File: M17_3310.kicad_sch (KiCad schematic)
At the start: 0 parts

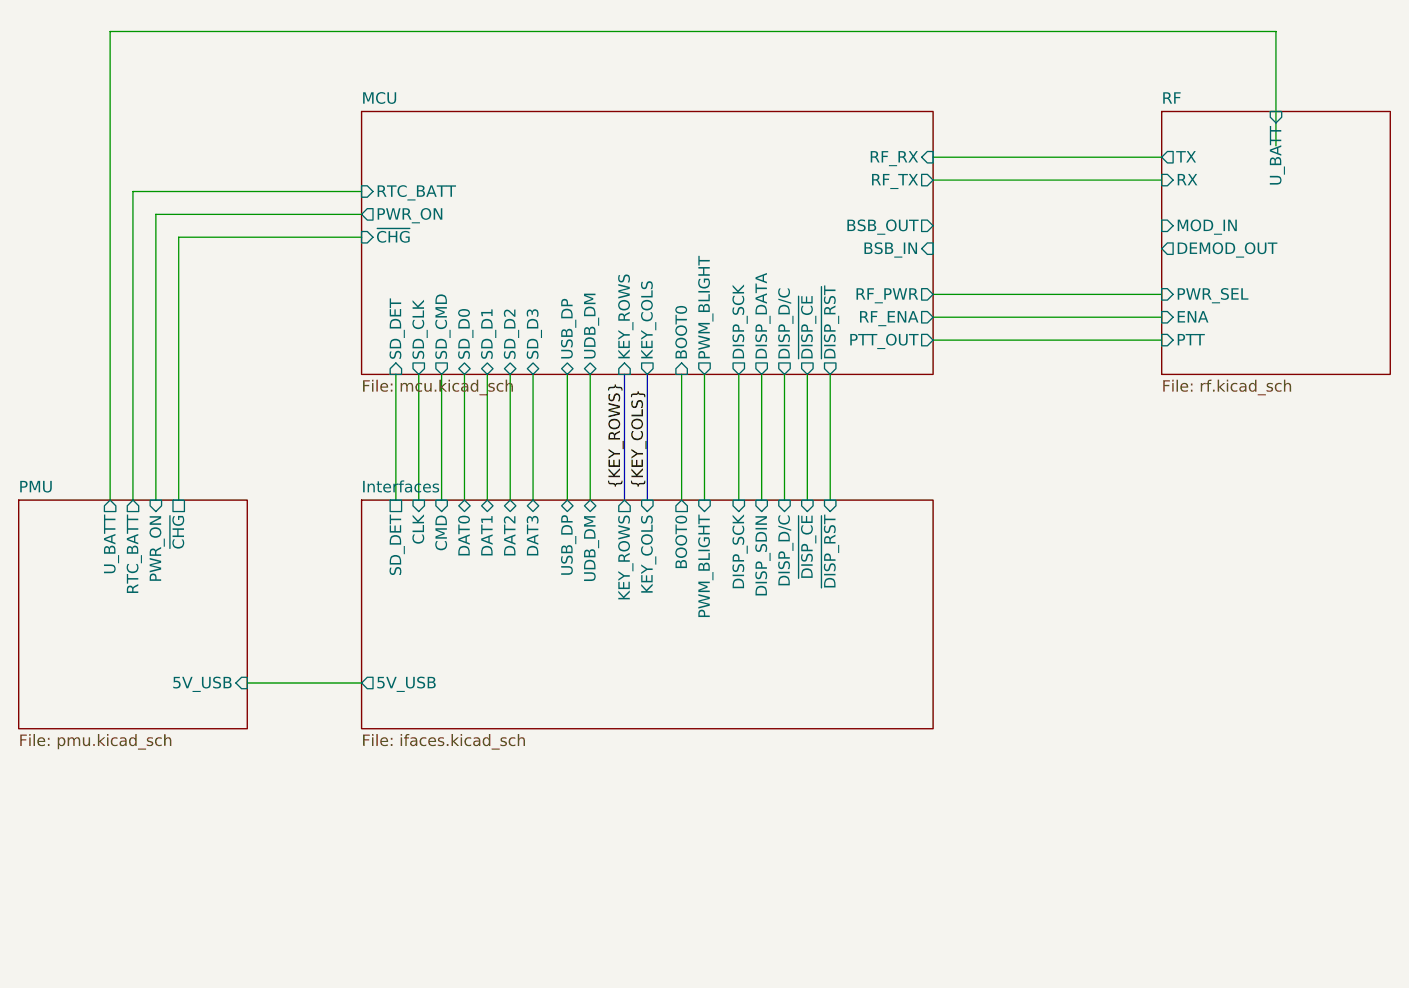
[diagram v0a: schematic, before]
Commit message: audio part
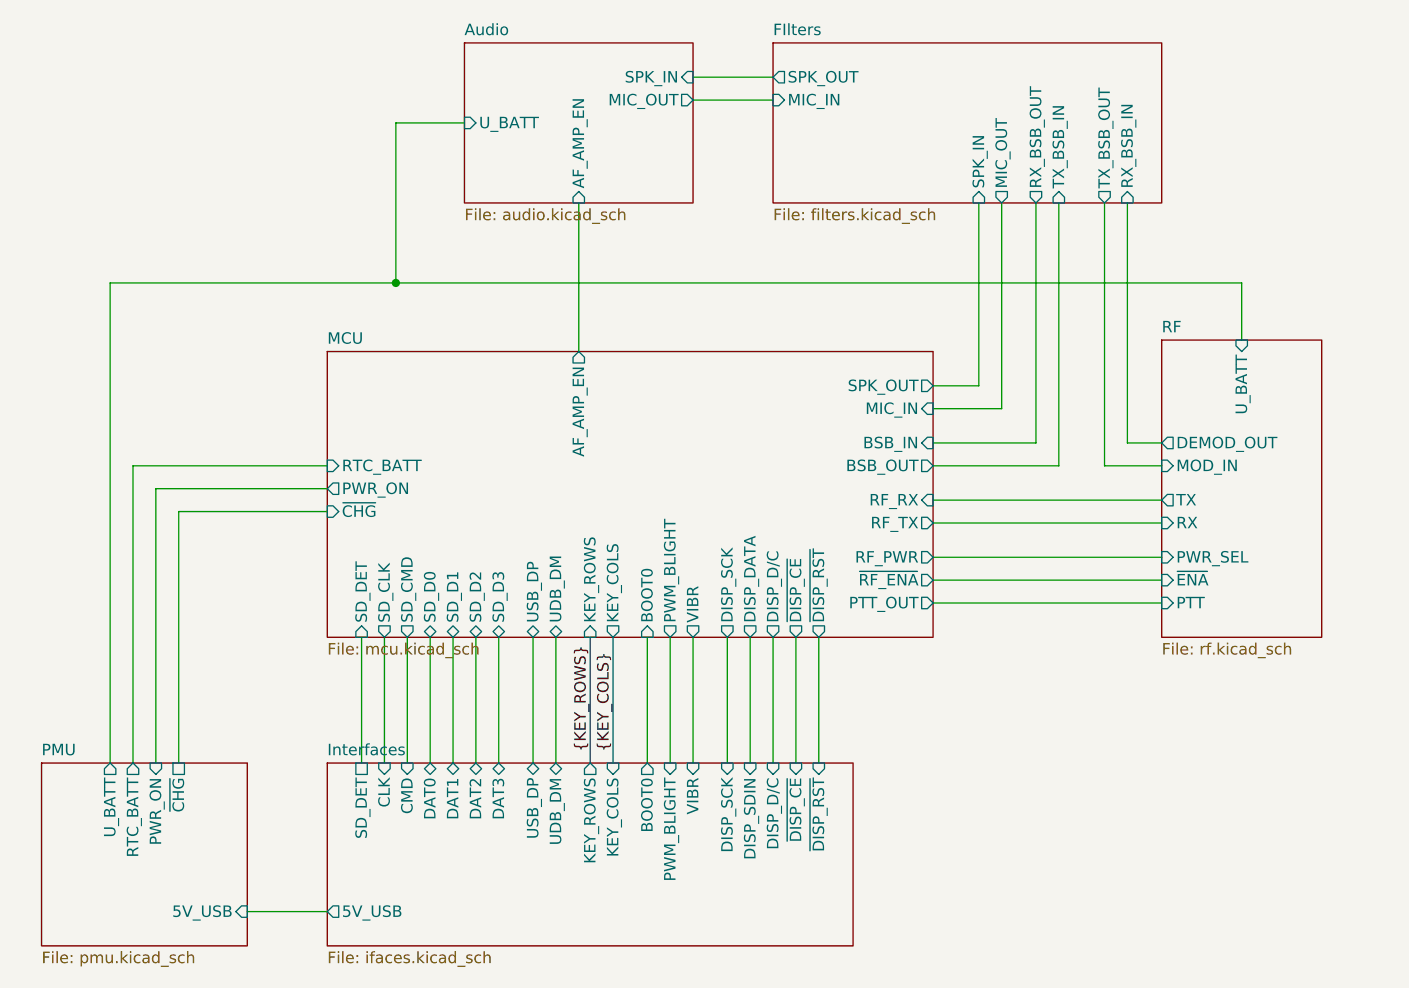
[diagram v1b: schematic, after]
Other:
- added sheet Audio (audio.kicad_sch)
- added sheet FIlters (filters.kicad_sch)
- sheet Interfaces ports: added VIBR; removed none
- sheet MCU ports: added AF_AMP_EN, MIC_IN, SPK_OUT, VIBR, ~{RF_ENA}; removed RF_ENA
- sheet RF ports: added ~{ENA}; removed ENA
